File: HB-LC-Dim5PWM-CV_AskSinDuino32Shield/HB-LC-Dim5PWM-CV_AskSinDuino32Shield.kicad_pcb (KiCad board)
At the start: 2 copper layers, 73.2 x 37.6 mm, 35 parts, among them J1 power+LED, J2 Encoder 1, J3 Encoder 2, Q11 IRF3708, Q12 IRF3708, Q13 IRF3708, Q14 IRF3708, U1 AskSinDuino32, U2 DS18B20, U3 LC78_05-0.5

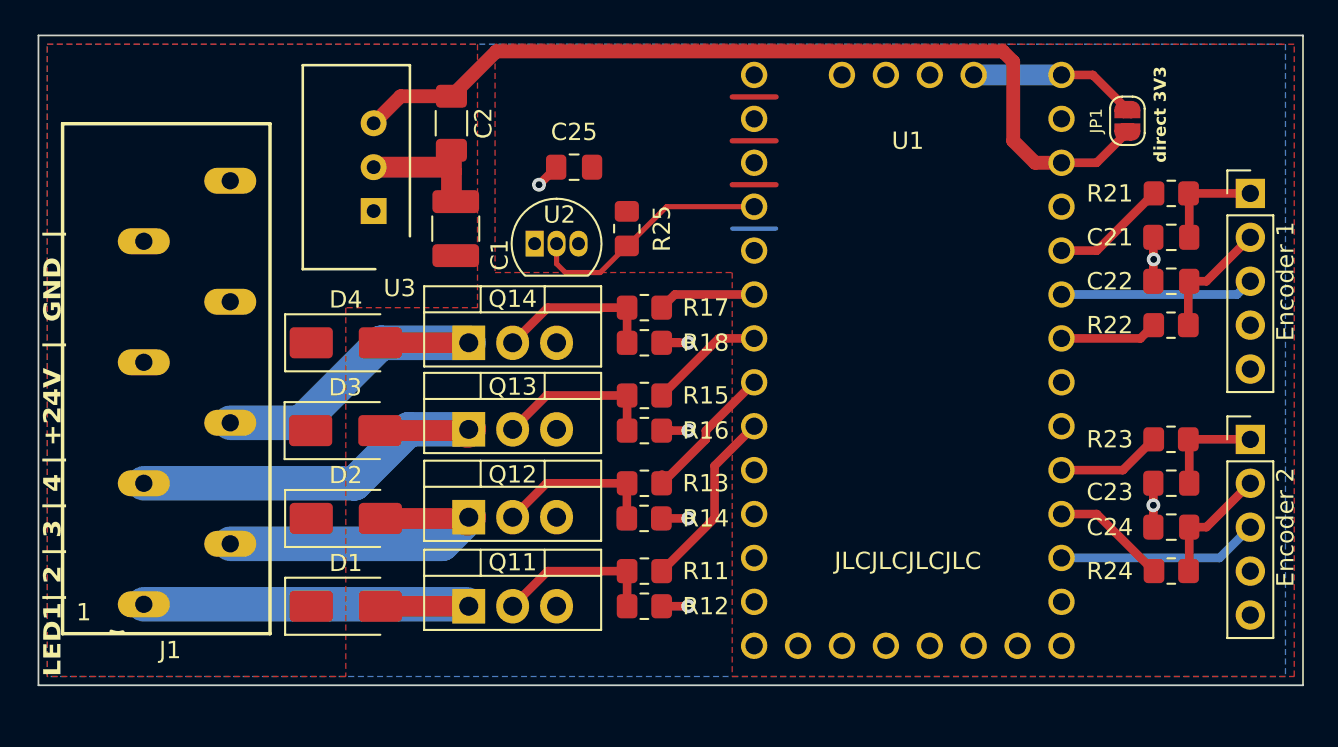
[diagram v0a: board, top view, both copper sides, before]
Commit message: HB-LC-Dim5PWM-CV_AskSinDuino32Shield
- 5th channel
- SMD FETs
- mounting holes
- PCB size and routing optimized
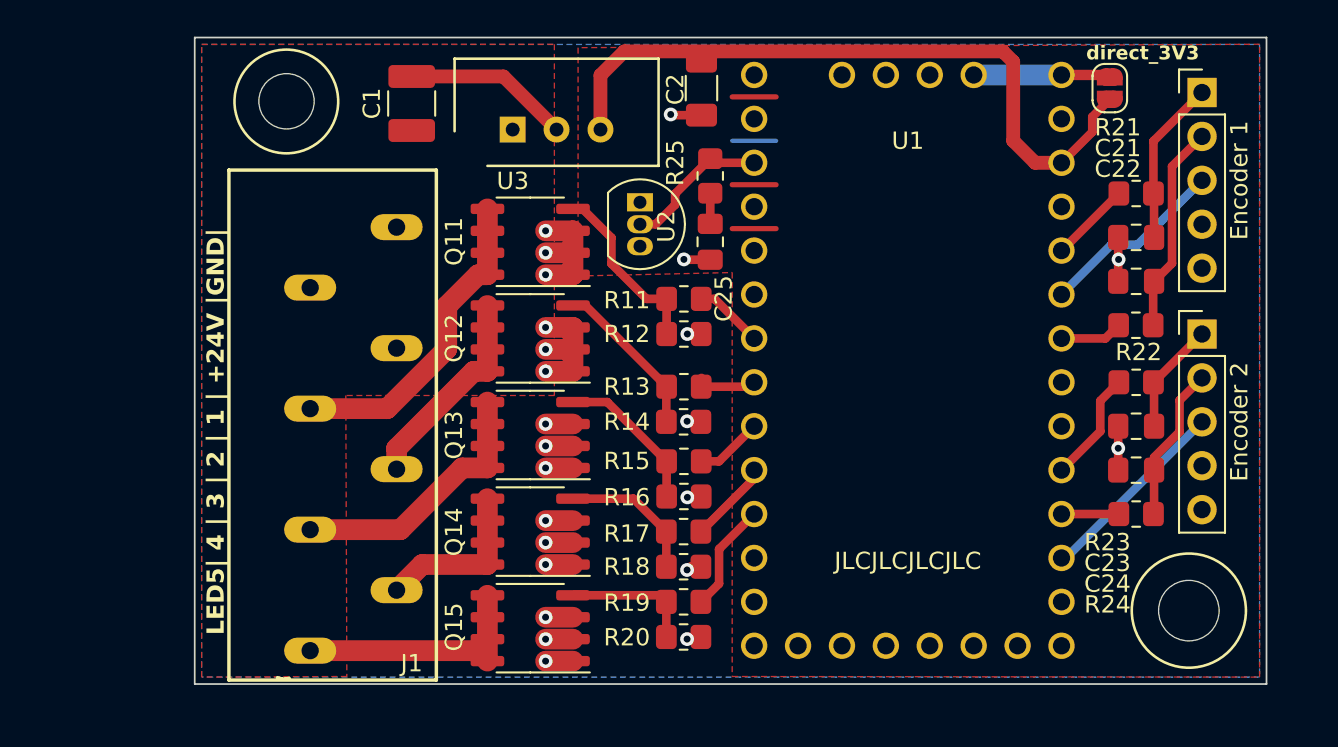
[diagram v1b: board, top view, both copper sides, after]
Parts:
- removed D1, D2, D3, D4: SS16, Diode_SMD:D_SMA
- added H1: MountingHole, MountingHole:MountingHole_3.2mm_M3, F.Cu at (100.7, 59.7)
- added H2: MountingHole, MountingHole:MountingHole_3.5mm, F.Cu at (152.9, 89.2)
- added Q15: IRF8788PbF, Package_SO:SOIC-8_3.9x4.9mm_P1.27mm, F.Cu at (114.8, 90.2)
- added R19: 100R, Resistor_SMD:R_0805_2012Metric_Pad1.20x1.40mm_HandSolder, F.Cu at (123.7, 88.6)
- added R20: 100k, Resistor_SMD:R_0805_2012Metric_Pad1.20x1.40mm_HandSolder, F.Cu at (123.7, 90.7)
- JP1: value direct 3V3 -> direct_3V3
- Q11, Q12, Q13, Q14: value IRF3708 -> IRF8788PbF; footprint Package_TO_SOT_THT:TO-220-3_Vertical -> Package_SO:SOIC-8_3.9x4.9mm_P1.27mm
- moved Q11 21.4 mm to (114.8, 67.8), turned to 180 degrees
- moved R12 15.9 mm to (123.7, 73.2)
- moved R11 15.9 mm to (123.7, 71.1)
- moved C2 14.6 mm to (124.7, 58.9)
- moved R18 13.2 mm to (123.7, 86.6)
- moved R17 13.2 mm to (123.7, 84.6)
- moved Q14 11.5 mm to (114.8, 84.6), turned to 180 degrees
- moved Q12 10.9 mm to (114.8, 73.4), turned to 180 degrees
- moved J1 9.99 mm to (103.4, 78.4)
- moved U3 9.32 mm to (113.8, 61.3), turned to 0 degrees
- moved C25 8.98 mm to (125.2, 67.8), turned to -90 degrees
- moved C1 7.67 mm to (108.0, 59.8)
- moved J3 6.71 mm to (153.7, 73.2)
- moved U2 6.55 mm to (121.2, 65.5), turned to -90 degrees
- moved J2 6.47 mm to (153.7, 59.2)
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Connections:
- J1 pad 1: /LED1 -> /LED5
- J1 pad 2: /LED2 -> /LED4
- J1 pad 4: /LED4 -> /LED2
- J1 pad 5: +24V -> /LED1
- J1 pad 7: GND -> +24V
- Q11 pad 1: /LED1 -> GND
- Q11 pad 2: Net-(Q11-G) -> GND
- Q12 pad 1: /LED2 -> GND
- Q12 pad 2: Net-(Q12-G) -> GND
- Q13 pad 1: /LED3 -> GND
- Q13 pad 2: Net-(Q13-G) -> GND
- Q14 pad 1: /LED4 -> GND
- Q14 pad 2: Net-(Q14-G) -> GND
- U1 pad W11: /1WIRE -> unconnected-(U1-PA2-PadW11)
- U1 pad W12: unconnected-(U1-PA1-PadW12) -> /1WIRE
- U1 pad W4: unconnected-(U1-PB1-PadW4) -> /PWM5
- U1 pad W5: unconnected-(U1-PB0-PadW5) -> /PWM4
- U1 pad W6: /PWM1 -> /PWM3
- U1 pad W8: /PWM3 -> /PWM1
- U1 pad W9: /PWM4 -> unconnected-(U1-PA4-PadW9)
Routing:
- net GND: track 32.1 -> 61.3 mm, vias 7 -> 24
- net /LED5: track 0.00 -> 14.3 mm
- net /LED4: track 20.8 -> 9.68 mm
- net +5V: track 51.4 -> 40.6 mm
- net /LED3: track 25.3 -> 15.5 mm
- net Net-(Q15-G): track 0.00 -> 7.59 mm
- net /LED2: track 19.6 -> 12.1 mm
- net /PWM1: track 10.6 -> 4.01 mm
- net /PWM5: track 0.00 -> 6.36 mm
- net /1WIRE: track 14.4 -> 8.65 mm
- net /LED1: track 24.1 -> 18.7 mm
- net Net-(J2-Pin_2): track 7.15 -> 12.3 mm
- net /PWM2: track 8.58 -> 3.69 mm
- net Net-(J2-Pin_1): track 6.13 -> 9.56 mm
- net /DATA2: track 6.72 -> 3.32 mm
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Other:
- board size 73.2 x 37.6 mm -> 62 x 37.4 mm
- board text added: "LED5| 4 | 3 | 2 | 1 | +24V |GND|"
- board text removed: "LED1| 2 | 3 | 4 | +24V | GND |"
